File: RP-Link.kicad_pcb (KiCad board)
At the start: 2 copper layers, 17 x 48.2 mm, 31 parts, among them J1 TYPE-C_16P, J2 Conn_01x06, SW1 SKRKAEE020_SMD, U1 W25Q16JVUX, U2 ME6211C33M5G, U3 RP2040, Y1 Crystal_GND24

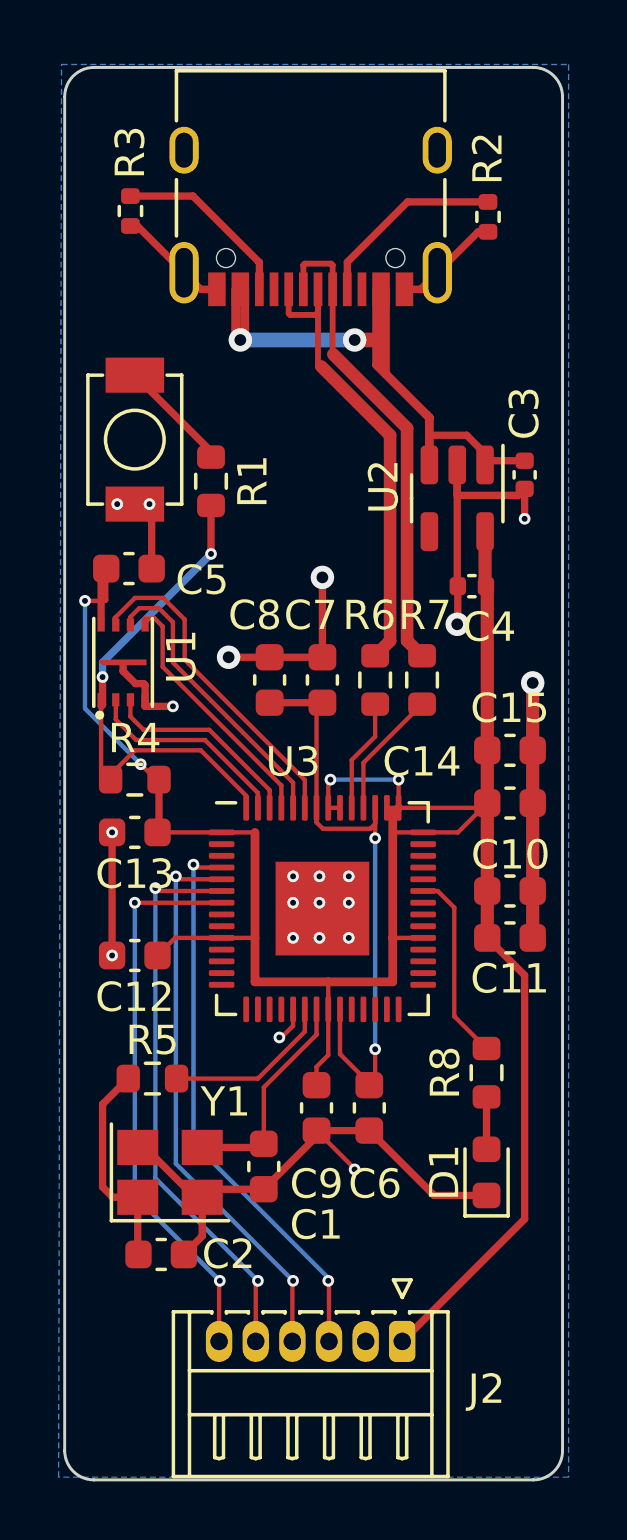
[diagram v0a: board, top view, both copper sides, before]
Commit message: 修复一些问题
#2
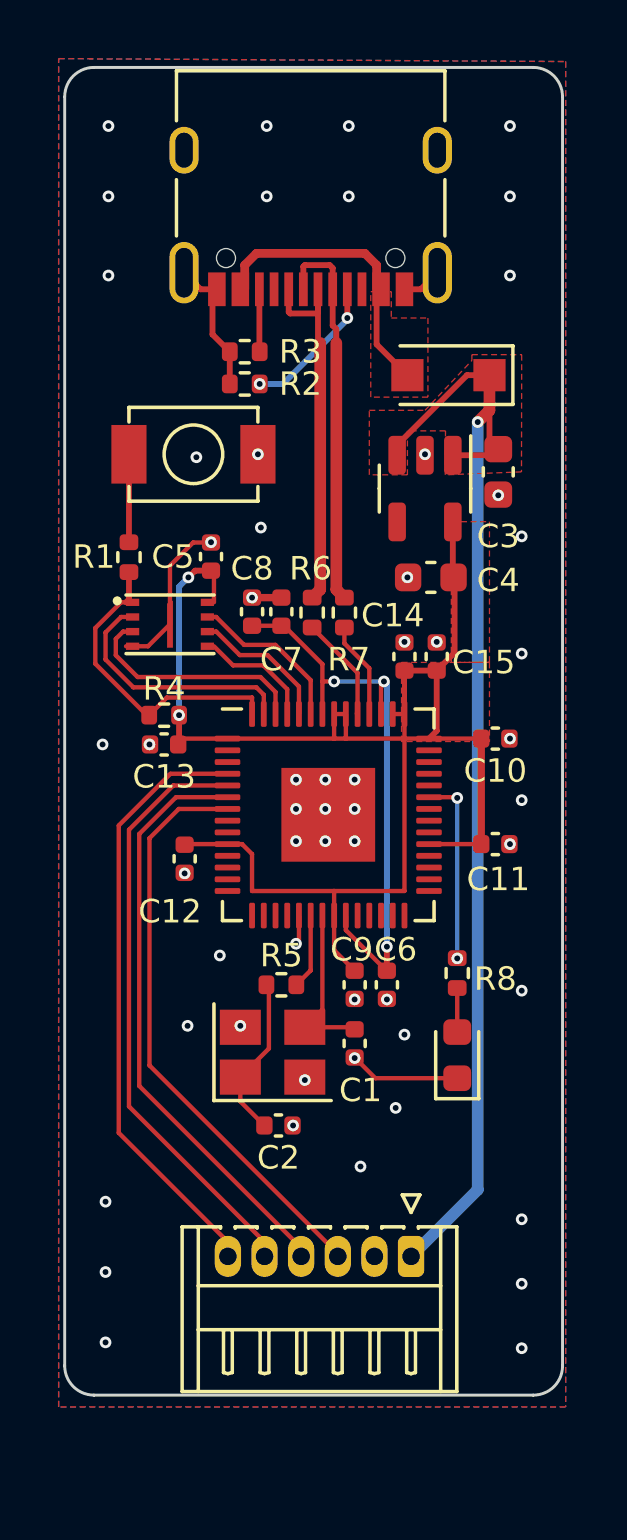
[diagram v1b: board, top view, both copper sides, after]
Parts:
- added D2: D_Schottky, Diode_SMD:D_SOD-123F, F.Cu at (129.3, 74.8)
- C1, C10, C11, C12, C13, C14, C15, C2, C5, C6, C7, C8, C9: footprint Capacitor_SMD:C_0603_1608Metric -> Capacitor_SMD:C_0402_1005Metric
- C3, C4: footprint Capacitor_SMD:C_0402_1005Metric -> Capacitor_SMD:C_0603_1608Metric
- R1, R4, R5, R6, R7, R8: footprint Resistor_SMD:R_0603_1608Metric -> Resistor_SMD:R_0402_1005Metric
- moved R2 10.1 mm to (122.3, 75.1), turned to 180 degrees
- moved R3 6.18 mm to (122.3, 74.0), turned to 180 degrees
- moved C14 6.16 mm to (127.8, 84.4), turned to 90 degrees
- moved C2 5.95 mm to (123.5, 100.4)
- moved R5 5.44 mm to (123.6, 95.6)
- moved Y1 5.39 mm to (123.3, 97.9)
- moved C10 5.22 mm to (130.9, 87.2)
- moved C1 5.22 mm to (126.1, 97.6)
- moved C9 4.40 mm to (126.1, 95.6)
- moved C6 4.24 mm to (127.2, 95.6)
- moved D1 4.12 mm to (129.6, 98.0)
- moved C15 4.06 mm to (128.9, 84.4), turned to 90 degrees
- moved R1 3.81 mm to (118.4, 81.0)
- moved C12 3.71 mm to (120.3, 91.3), turned to -90 degrees
- moved R8 3.54 mm to (129.6, 95.2)
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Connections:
- C3 pad 1: VBUS -> VCC
- J2 pad 1: +3.3V -> VCC
- J2 pad 3: /GPIO2 -> /GPIO5
- J2 pad 4: /GPIO3 -> /GPIO4
- J2 pad 5: /GPIO4 -> /GPIO3
- J2 pad 6: /GPIO5 -> /GPIO2
- U2 pad 1: VBUS -> VCC
- U2 pad 3: VBUS -> VCC
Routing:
- net GND: track 61.4 -> 17.3 mm, vias 21 -> 56
- net VCC: track 0.00 -> 39.9 mm, vias 0 -> 1
- net +3.3V: track 81.8 -> 55.5 mm, vias 4 -> 2
- net VBUS: track 24.9 -> 10.4 mm, vias 2 -> 0
- net /QSPI_SS: track 17.2 -> 10.6 mm, vias 2 -> 0
- net /QSPI_SD3: track 11.1 -> 5.35 mm
- net /QSPI_SCLK: track 9.85 -> 4.62 mm
- net /QSPI_SD0: track 8.58 -> 3.95 mm
- net Net-(J1-PadB5): track 6.25 -> 2.13 mm
- net /XIN: track 5.80 -> 2.57 mm
- net /USB_D-: track 16.5 -> 13.2 mm
- net /USB_D+: track 16.5 -> 13.5 mm
- net Net-(C2-Pad2): track 7.37 -> 5.58 mm
- net /XOUT: track 7.48 -> 5.79 mm
- net Net-(J1-PadA5): track 6.58 -> 4.93 mm, vias 0 -> 2
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- added copper zone on F.Cu, net +3.3V
- added copper zone on F.Cu, net GND
- added copper zone on F.Cu, net VBUS
- added copper zone on F.Cu, net VCC
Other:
- board size 17 x 48.2 mm -> 17 x 45.3 mm
